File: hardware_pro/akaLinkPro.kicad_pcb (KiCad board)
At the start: 2 copper layers, 45 x 45 mm, 96 parts, among them J1 USB_C_Receptacle_USB2.0_16P, J101 Conn_02x05_Odd_Even, J103 IDC, J2 ISP, Q1 SI2305, Q104 AO3400A, SW101 BL, U1 XC6206P332MR, U101 HPM5301IEG1, U102 USBLC6-2SC6, U103 SN74LVC1T45DBV, U105 TPS22918DBV, U110 SN74LVC1T45DBV, U111 SN74LVC1T45DBV, U112 SN74LVC1T45DBV, U113 SN74LVC1T45DBV, U2 LMV321, U3 SN74LVC1T45DBV, Y101 24MHz

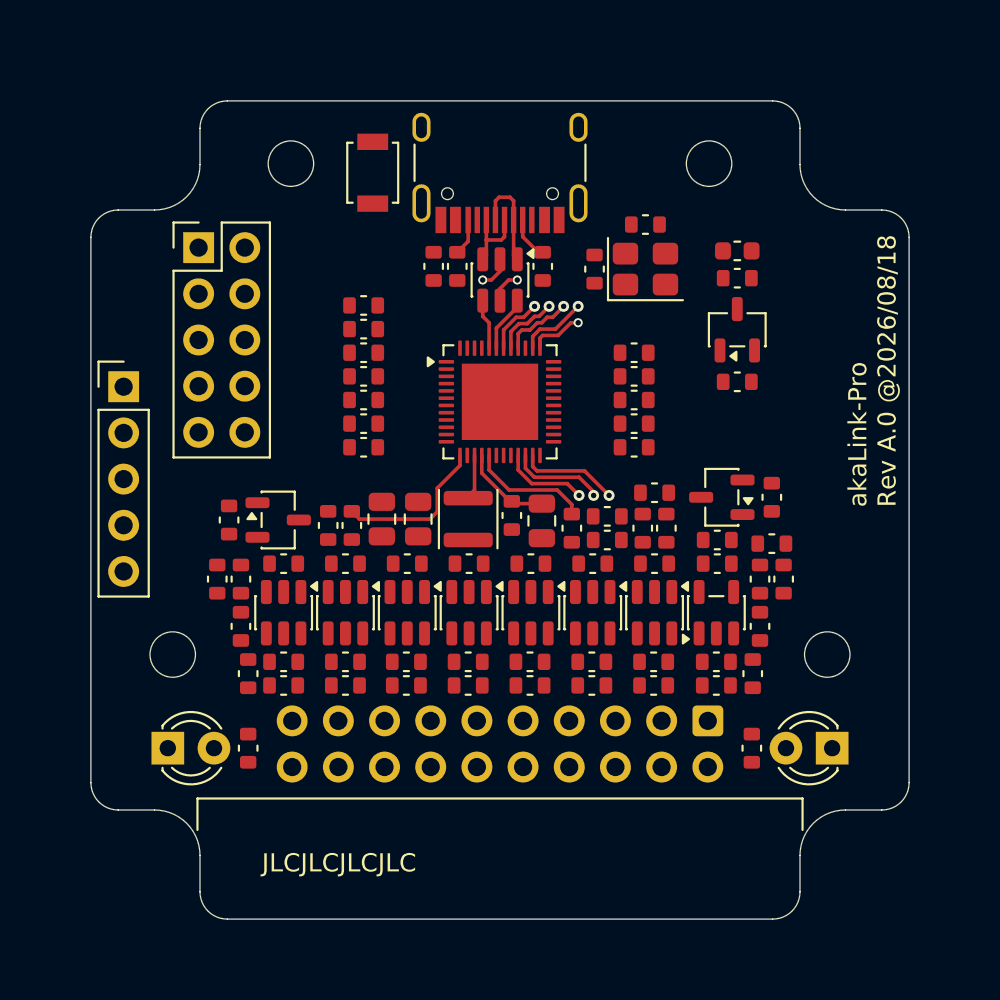
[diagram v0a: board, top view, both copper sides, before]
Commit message: update pcb
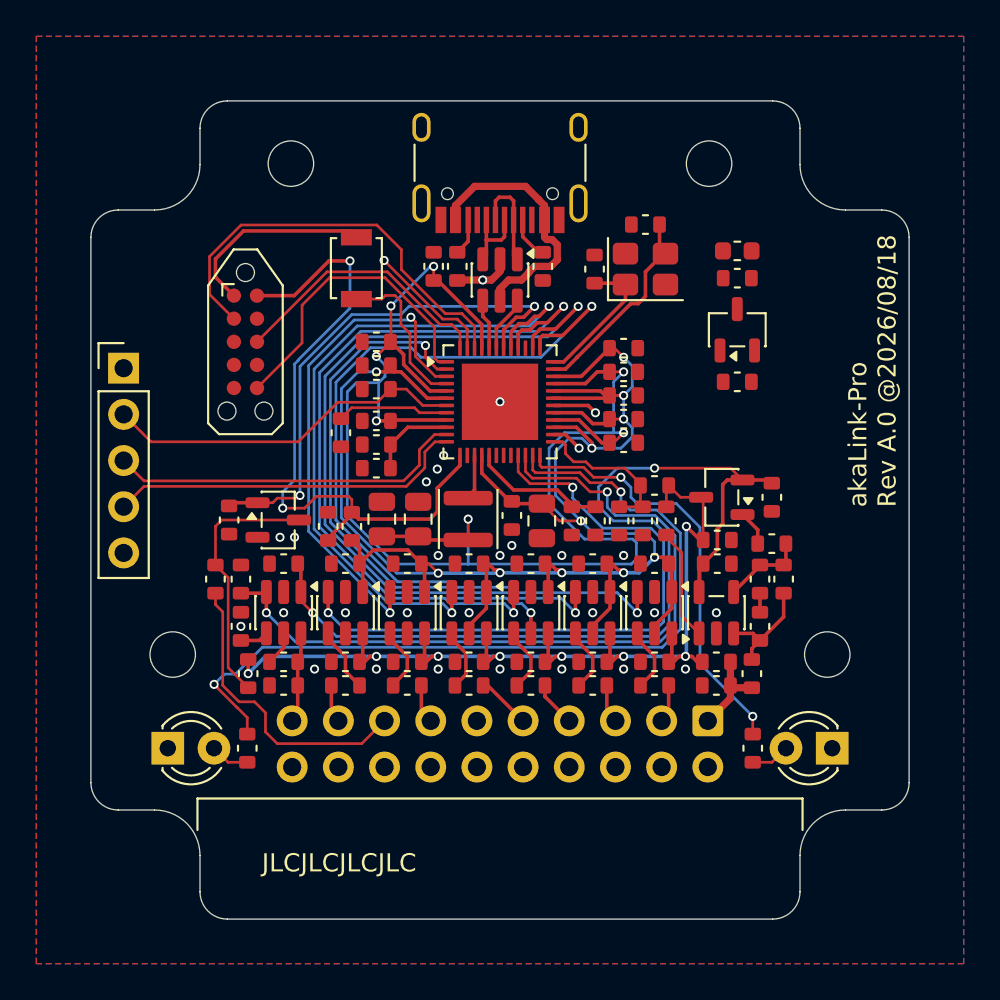
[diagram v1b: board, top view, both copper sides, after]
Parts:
- removed J101: Conn_02x05_Odd_Even, Connector_PinHeader_2.54mm:PinHeader_2x05_P2.54mm_Vertical
- added J3: TC2050, Connector:Tag-Connect_TC2050-IDC-NL_2x05_P1.27mm_Vertical, F.Cu at (57.5, 139.8)
- moved R104 5.84 mm to (62.8, 144.8), turned to -90 degrees
- moved SW101 5.33 mm to (63.6, 135.8)
- moved R103 4.65 mm to (64.7, 142.4)
- moved C105 1.35 mm to (64.7, 146.8)
- moved C117 1.35 mm to (64.7, 144.2)
- moved C106 1.35 mm to (64.7, 145.4)
- moved C121 1.30 mm to (62.0, 149.9), turned to 90 degrees
- moved R101 1.30 mm to (63.4, 149.9)
- moved C1 1.23 mm to (78.0, 149.7), turned to -90 degrees
- moved J2 1.02 mm to (50.8, 141.2)
- moved C118 0.92 mm to (64.7, 139.8)
- moved C129 0.92 mm to (64.7, 141.1)
- moved C108 0.70 mm to (76.8, 149.7), turned to -90 degrees
- moved C109 0.63 mm to (78.3, 142.8)
- moved C115 0.63 mm to (78.3, 141.4)
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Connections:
- J2 pad 3: /ISP_TX -> /ISP_RX
- J2 pad 4: /ISP_RX -> /ISP_TX
- U101 pad 22: /LED2 -> /5V_EN
- U101 pad 23: /LED1 -> /LED2
- U101 pad 24: /ADC_VREF -> /LED1
- U101 pad 25: /5V_EN -> /ADC_VREF
- U101 pad 47: /DBG_JTCK -> GND
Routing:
- net +3V3: track 4.97 -> 118.8 mm, vias 0 -> 11
- net VDD_SOC: track 0.00 -> 85.2 mm, vias 0 -> 7
- net VEE: track 0.00 -> 56.5 mm, vias 0 -> 8
- net +5V: track 0.00 -> 51.9 mm, vias 0 -> 2
- net /JTRST: track 3.01 -> 47.8 mm, vias 1 -> 2
- net /5V_EN: track 0.00 -> 42.1 mm, vias 0 -> 2
- net /LED2: track 5.19 -> 46.3 mm, vias 1 -> 2
- net /JTMS_DIR: track 3.83 -> 42.0 mm, vias 1 -> 2
- net /JTMS_IN: track 3.92 -> 41.1 mm, vias 1 -> 2
- net /JTCK: track 3.59 -> 37.4 mm, vias 1 -> 2
- net /JTDI_TXD: track 0.00 -> 32.7 mm, vias 0 -> 2
- net /AUX_RXD: track 4.73 -> 35.4 mm, vias 1 -> 2
- net /nRST: track 8.66 -> 36.6 mm, vias 0 -> 2
- net /JTDO_RXD: track 0.00 -> 27.7 mm, vias 0 -> 2
- net /nRESET: track 3.24 -> 28.7 mm, vias 1 -> 2
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- added copper zone on B.Cu, net GND
- added copper zone on F.Cu, net GND
